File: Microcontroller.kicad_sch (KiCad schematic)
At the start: 33 parts, among them SW1 KMR221GLFS, U4 STM32F446RET6, U7 W25Q128JVSIQ, Y1 16MHz

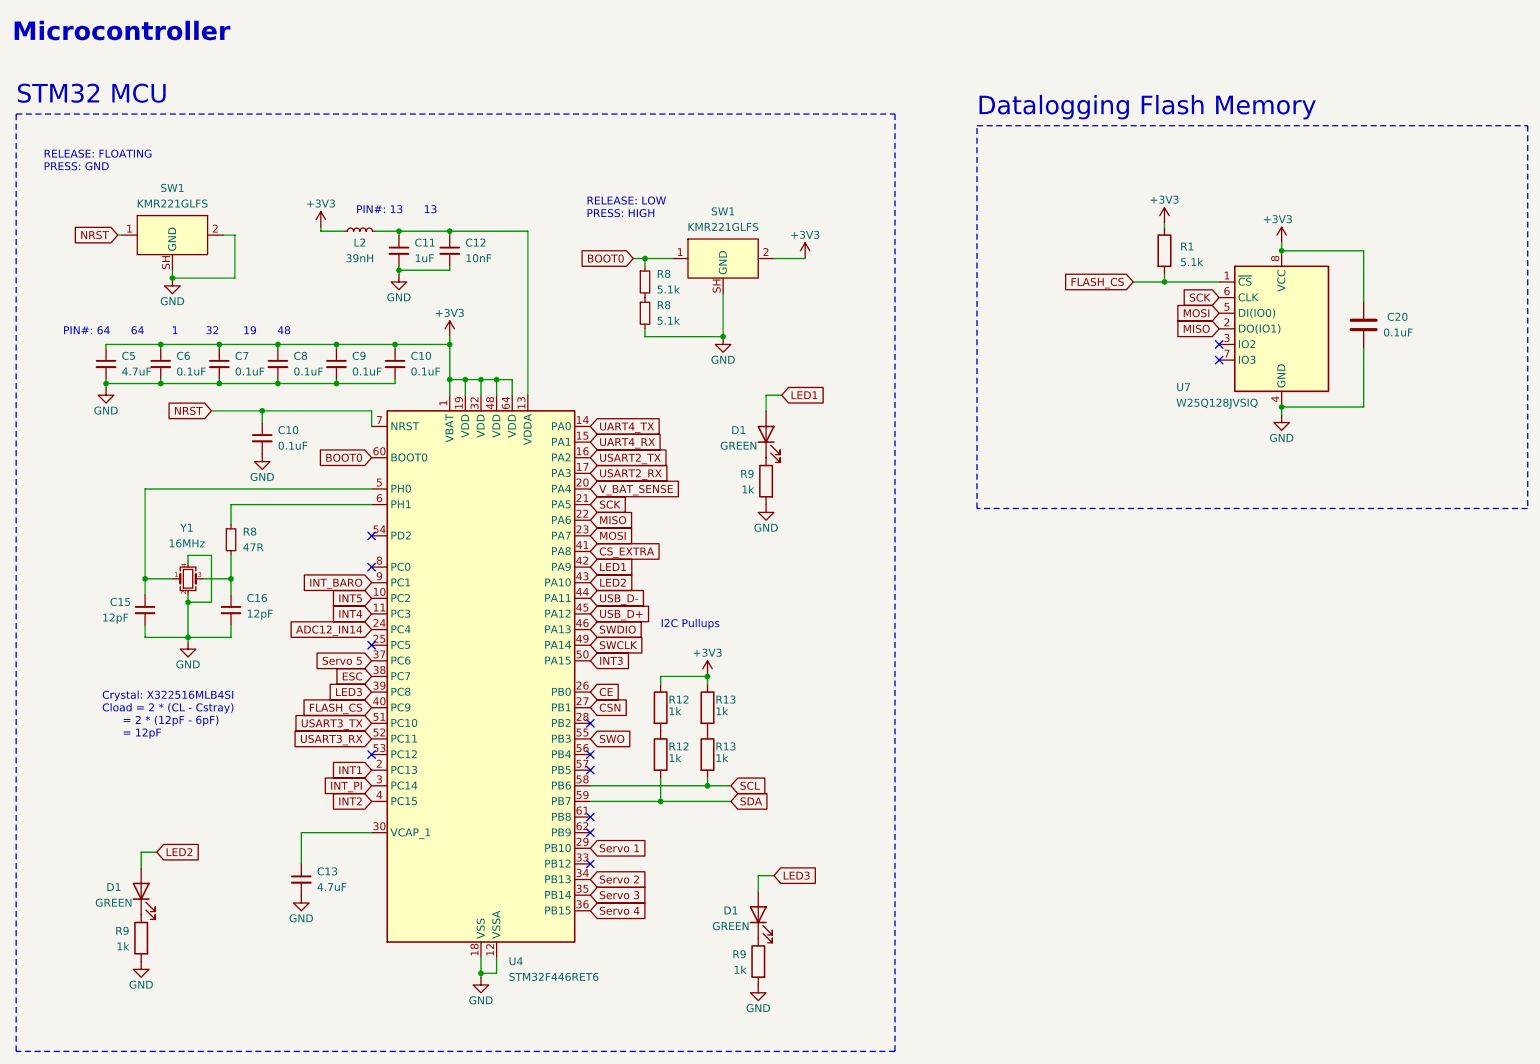
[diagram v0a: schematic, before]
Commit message: Add files via upload
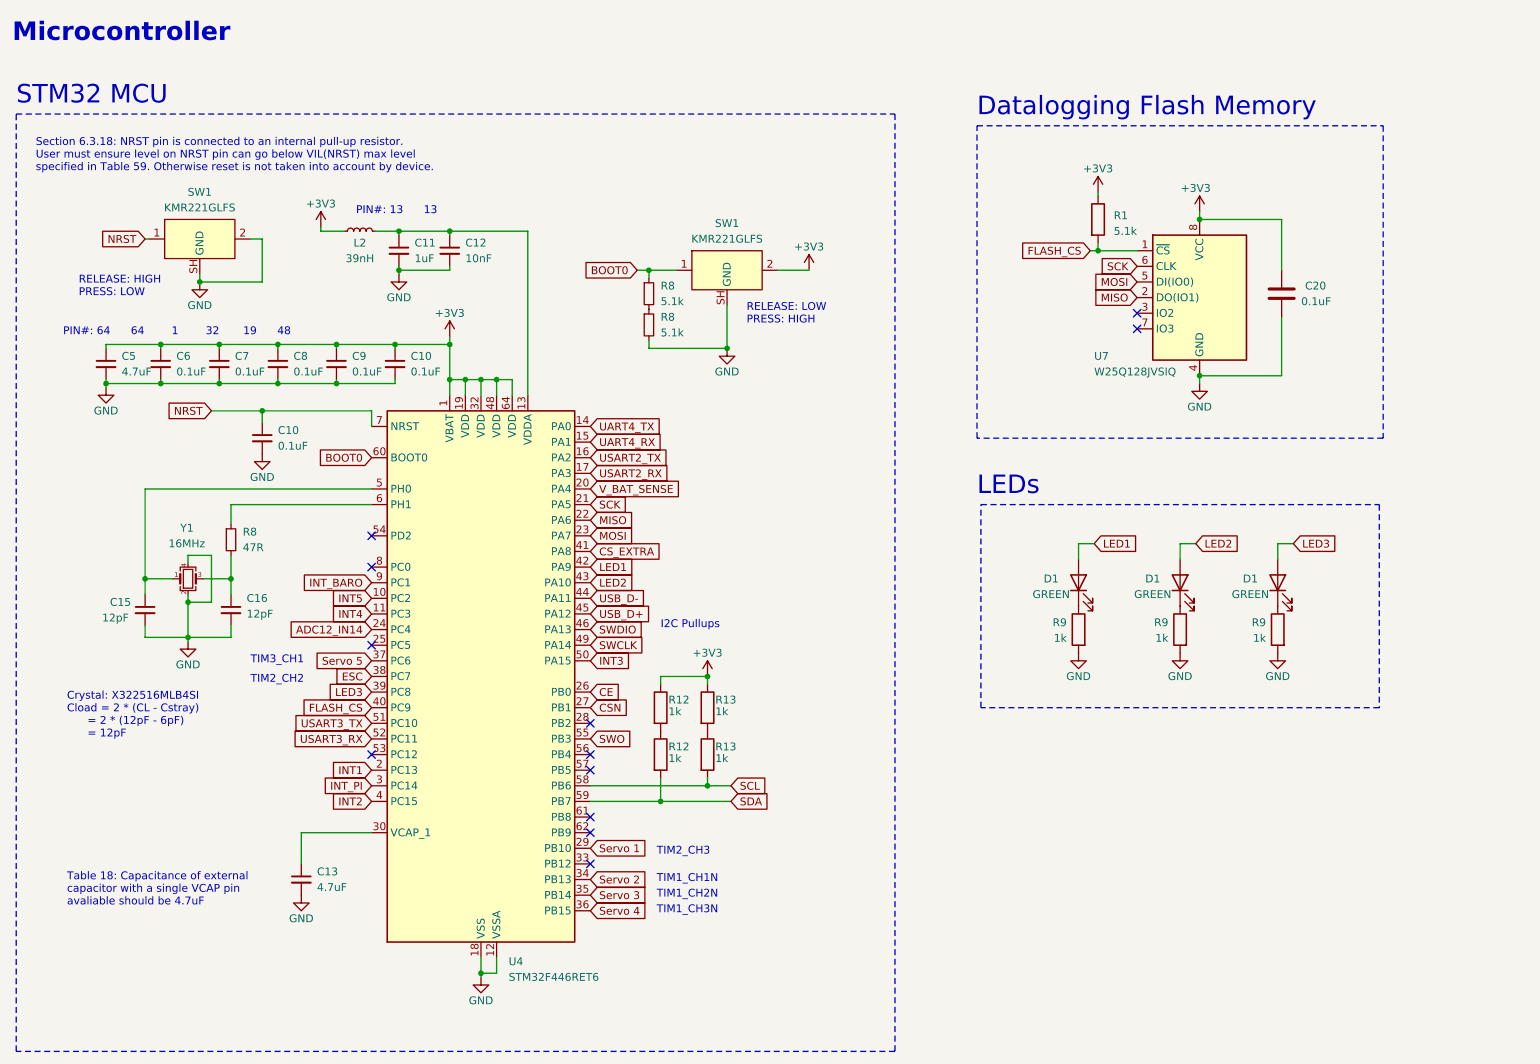
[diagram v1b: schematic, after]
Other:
- note added: "LEDs"
- note added: "RELEASE: HIGH PRESS: LOW"
- note added: "Section 6.3.18: NRST pin is connected to an internal pull-up resistor. User must ensure level on NRST pin can go below VIL(NRST) max level specified in Table 59. Otherwise reset is not taken into account by device."
- note added: "TIM1_CH1N"
- note added: "TIM1_CH2N"
- note added: "TIM1_CH3N"
- note added: "TIM2_CH2"
- note added: "TIM2_CH3"
- note added: "TIM3_CH1"
- note added: "Table 18: Capacitance of external capacitor with a single VCAP pin avaliable should be 4.7uF"
- note removed: "RELEASE: FLOATING PRESS: GND"
- moved on the sheet: C20, D1, R1, R8, R9, SW1, U7
